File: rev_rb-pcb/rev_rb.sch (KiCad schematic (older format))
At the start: 35 parts, among them CON1 BARREL_JACK, Q1 MOSFET-PCHANNELSMD, Q2 MOSFET-NCHANNELSMD, U1 STM32F103RB, U2 PC817, U3 PC817, Y1 8Mhz, Y2 32kHz

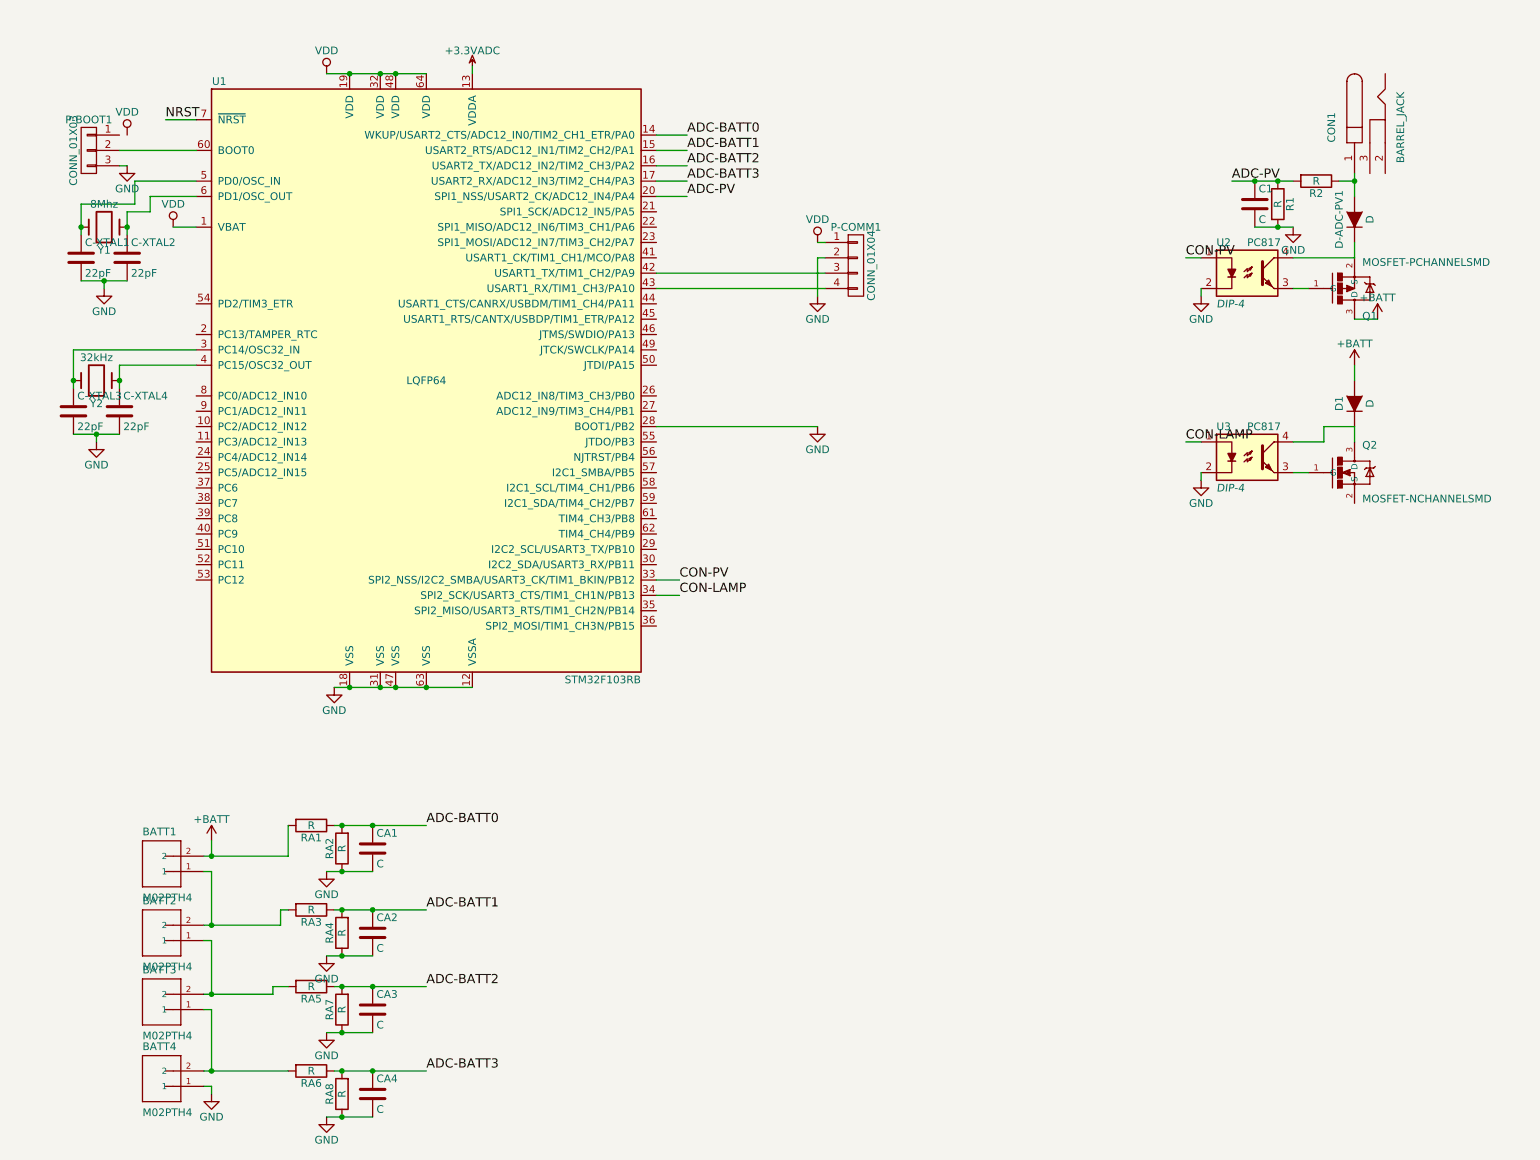
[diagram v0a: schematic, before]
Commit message: next gen PSHS
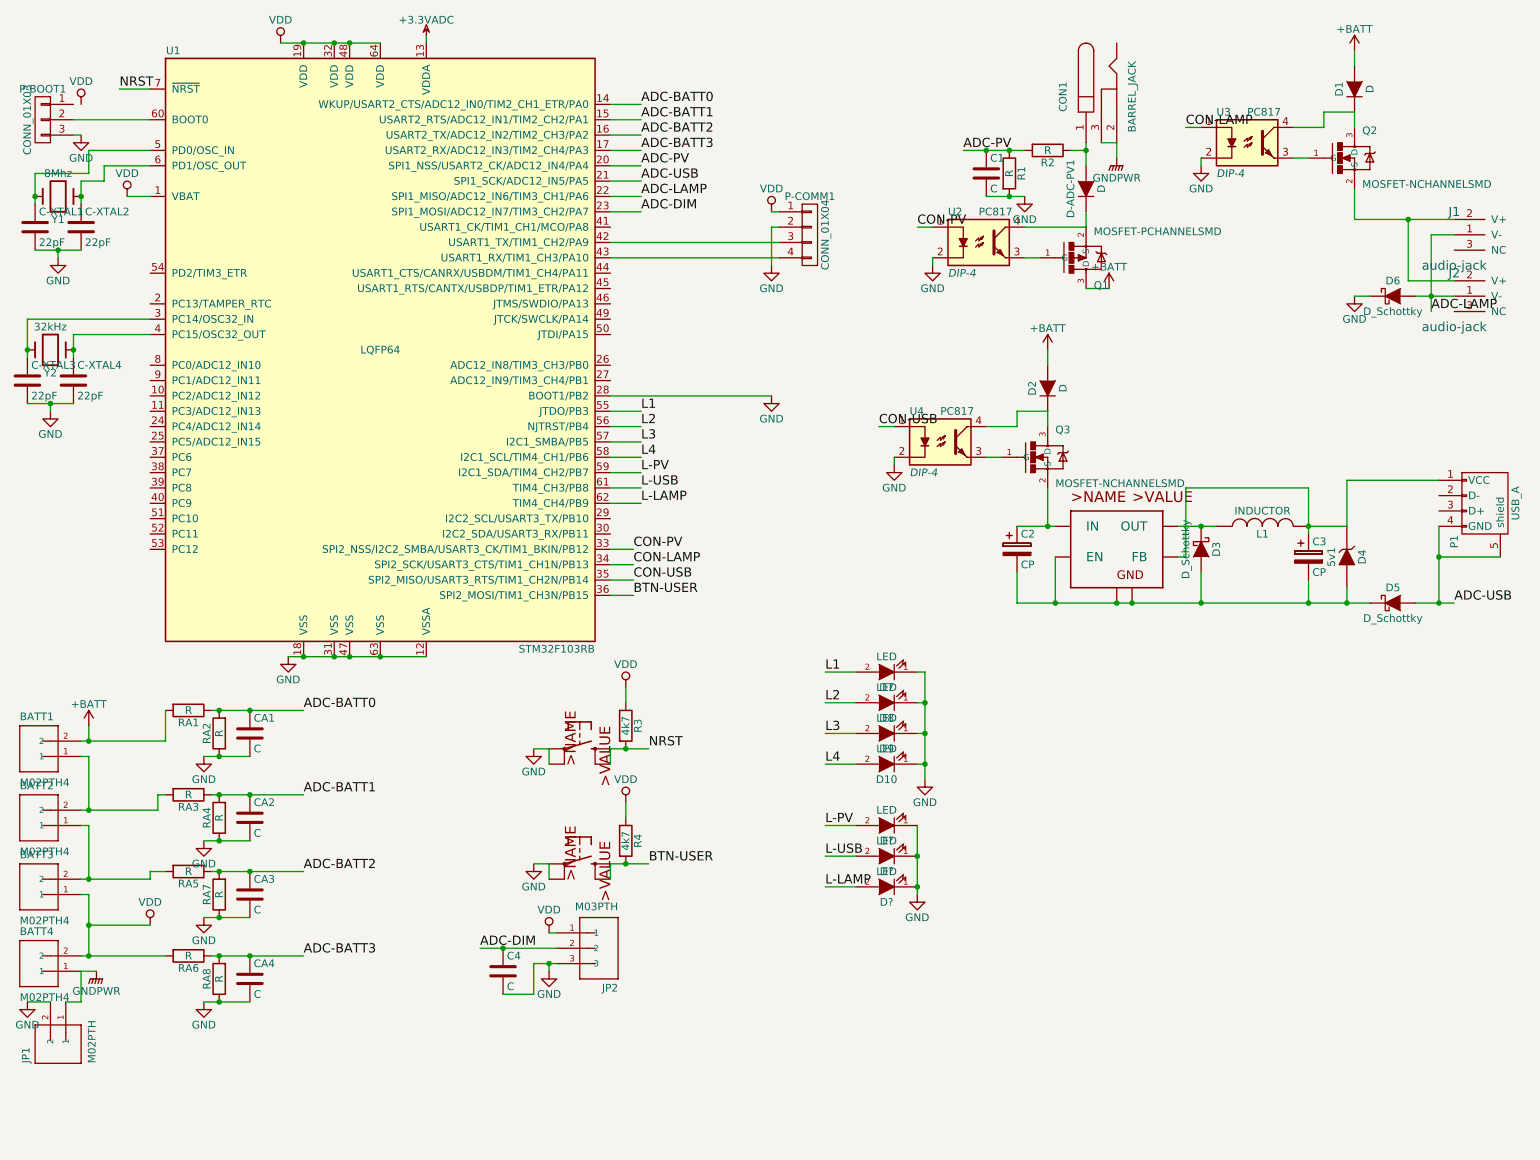
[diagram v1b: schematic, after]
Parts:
- added C2, C3: CP, symbol CP
- added C4: C, symbol C
- added D10, D7, D8, D9, D? (x3): LED, symbol LED
- added D2: D, symbol D
- added D3, D5, D6: D_Schottky, symbol D_Schottky
- added D4: 5v1, symbol ZENER
- added J1, J2: audio-jack, symbol audio-jack
- added JP1: M02PTH, SparkFun-1X02, symbol M02PTH
- added JP2: M03PTH, SparkFun-1X03, symbol M03PTH
- added L1: INDUCTOR, symbol INDUCTOR
- added P1: USB_A, symbol USB_A
- added Q3: MOSFET-NCHANNELSMD, SparkFun-SOT23-3, symbol MOSFET-NCHANNELSMD
- added R3, R4: 4k7, symbol R
- added U4: PC817, DIP-4, symbol PC817
- added U5: LM2596S_TO263-5, symbol LM2596S_TO263-5
- added U6: 10-XX_B3F-10XX, symbol 10-XX_B3F-10XX
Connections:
- net +BATT: now also D2.2 (A)
- net GND: now also C4.2, D10.1 (K), D6.1 (K), D7.1 (K), D8.1 (K), D9.1 (K), D?.1 (K), D?.1 (K), D?.1 (K), JP1.2, JP2.3, U4.2, U6.3 (P), U6.3 (P), U6.4 (P1), U6.4 (P1); no longer BATT4.1
- net NRST: now also R3.2, U6.1 (S), U6.2 (S1)
- net VDD: now also BATT3.1, BATT4.2, RA6.2, JP2.1, R3.1, R4.1
- net ADC-USB: now reaches U1.21 (SPI1_SCK/ADC12_IN5/PA5)
- net ADC-USB: now also D5.2 (A), P1.4 (GND), P1.5 (shield)
- net ADC-LAMP: now reaches U1.22 (SPI1_MISO/ADC12_IN6/TIM3_CH1/PA6)
- net ADC-LAMP: now also D6.2 (A), J1.1 (V-), J2.1 (V-)
- net ADC-DIM: now reaches U1.23 (SPI1_MOSI/ADC12_IN7/TIM3_CH2/PA7)
- net ADC-DIM: now also C4.1, JP2.2
- net CON-USB: now reaches U1.35 (SPI2_MISO/USART3_RTS/TIM1_CH2N/PB14)
- net CON-USB: now also U4.1
- net BTN-USER: now reaches U1.36 (SPI2_MOSI/TIM1_CH3N/PB15)
- net BTN-USER: now also R4.2, U6.1 (S), U6.2 (S1)
- net L1: now reaches U1.55 (JTDO/PB3)
- net L1: now also D7.2 (A)
- net L2: now reaches U1.56 (NJTRST/PB4)
- net L2: now also D8.2 (A)
- net L3: now reaches U1.57 (I2C1_SMBA/PB5)
- net L3: now also D9.2 (A)
- net L4: now reaches U1.58 (I2C1_SCL/TIM4_CH1/PB6)
- net L4: now also D10.2 (A)
- net L-PV: now reaches U1.59 (I2C1_SDA/TIM4_CH2/PB7)
- net L-PV: now also D?.2 (A)
- net L-USB: now reaches U1.61 (TIM4_CH3/PB8)
- net L-USB: now also D?.2 (A)
- net L-LAMP: now reaches U1.62 (TIM4_CH4/PB9)
- net L-LAMP: now also D?.2 (A)
- net GNDPWR: now reaches CON1.2
- net GNDPWR: now also BATT4.1, CON1.3, JP1.1
- net at Q2.2 (S): now also J1.2 (V+), J2.2 (V+)
- new net: Q3.1 (G), U4.3
- new net: C2.1, Q3.2 (S), U5.1 (IN)
- new net: D2.1 (K), Q3.3 (D), U4.4
- new net: D3.1 (K), L1.1, U5.2 (OUT)
- new net: C2.2, C3.2, D3.2 (A), D4.2 (A), D5.1 (K), U5.3 (GND), U5.5 (EN), U5.6 (GND@1)
- new net: C3.1, D4.1 (K), L1.2, P1.1 (VCC), U5.4 (FB)
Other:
- moved on the sheet: BATT1, BATT2, BATT3, BATT4, C-XTAL1, C-XTAL2, C-XTAL3, C-XTAL4, C1, CA1, CA2, CA3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
